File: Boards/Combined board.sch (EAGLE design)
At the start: 9 parts

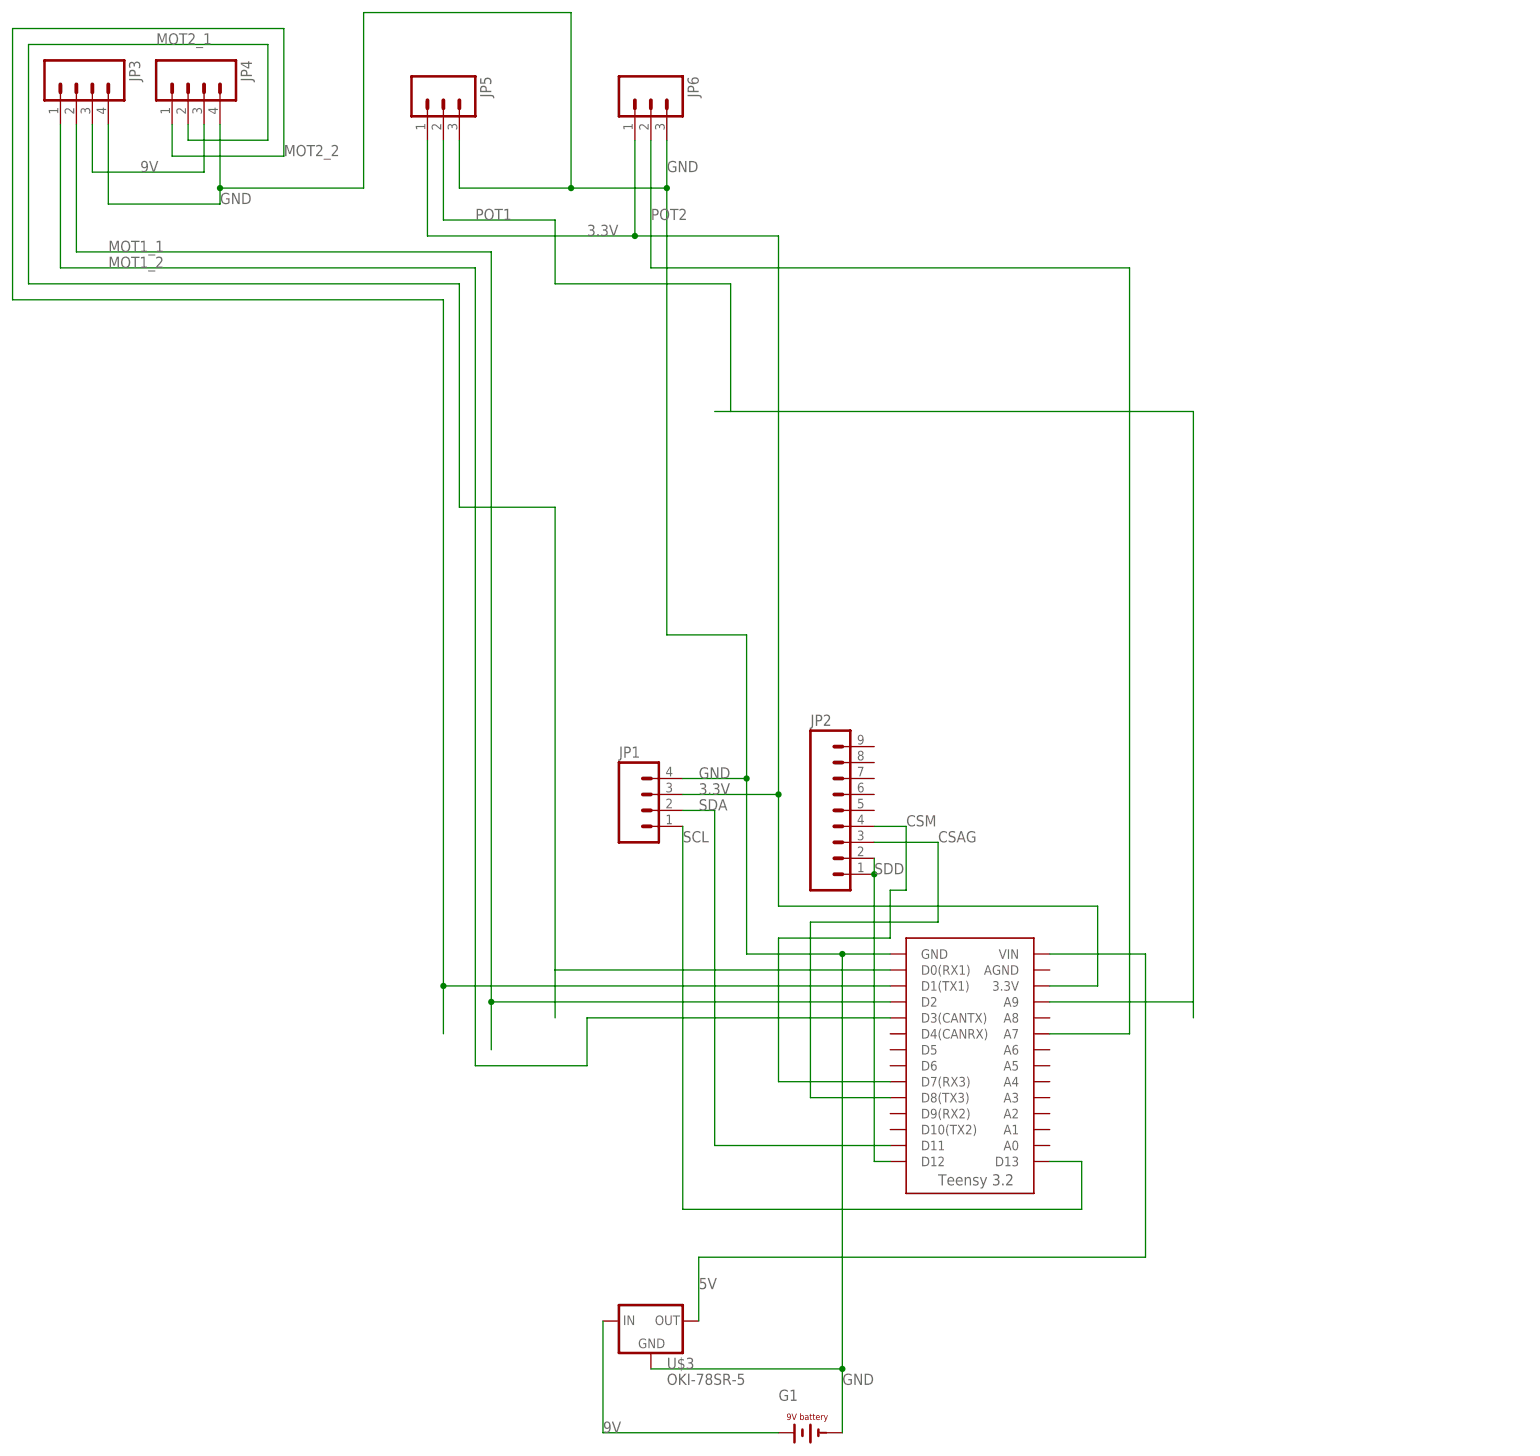
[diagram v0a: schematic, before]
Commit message: Final Push
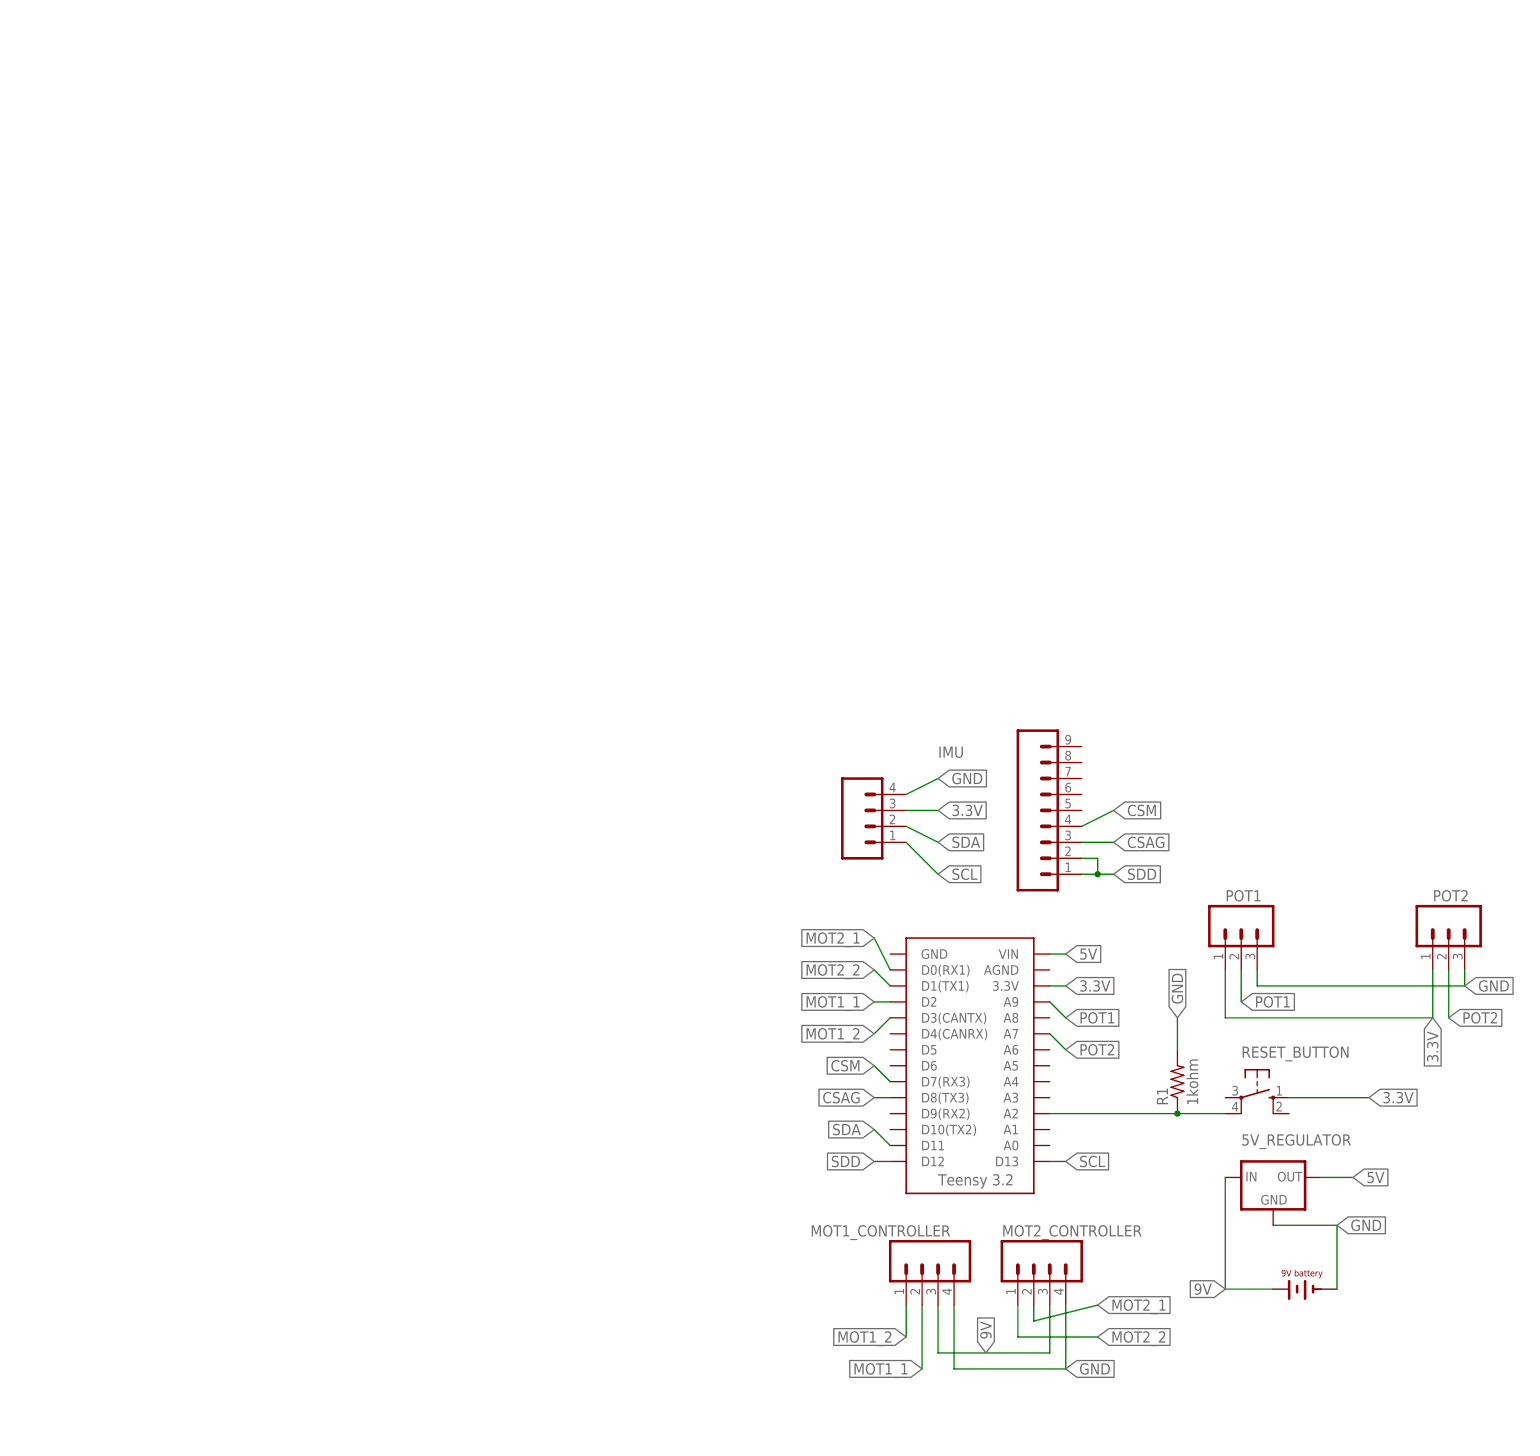
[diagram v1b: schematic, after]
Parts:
- removed JP2: (no value), HyTechDevices:M09
- removed JP3, JP4: (no value), HyTechDevices:M04
- removed JP5, JP6: (no value), HyTechDevices:M03
- removed U$3: OKI-78SR-5, HyTechDevices:OKI-78SR-5
- added 5V_REGULATOR: OKI-78SR-5, HyTechDevices:OKI-78SR-5
- added IMU: (no value), HyTechDevices:M09
- added MOT1_CONTROLLER, MOT2_CONTROLLER: (no value), HyTechDevices:M04
- added POT1, POT2: (no value), HyTechDevices:M03
- added R1: 1kohm, HyTechDevices:RESISTORAXIAL-0.3
- added RESET_BUTTON: (no value), HyTechDevices:BTN_10-XX
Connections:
- new net N$1: R1.1, RESET_BUTTON.P1, U$2.A2
- net 3.3V: now also POT1.1, POT2.1, RESET_BUTTON.S; no longer JP5.1, JP6.1
- net 5V: now also 5V_REGULATOR.OUT; no longer U$3.OUT
- net 9V: now also 5V_REGULATOR.IN, MOT1_CONTROLLER.3, MOT2_CONTROLLER.3; no longer JP3.3, JP4.3, U$3.IN
- net CSAG: now also IMU.3; no longer JP2.3
- net CSM: now also IMU.4; no longer JP2.4
- net GND: now also 5V_REGULATOR.GND, MOT1_CONTROLLER.4, MOT2_CONTROLLER.4, POT1.3, POT2.3, R1.2; no longer JP3.4, JP4.4, JP5.3, JP6.3, U$2.GND, U$3.GND
- net MOT1_1: now also MOT1_CONTROLLER.2; no longer JP3.2
- net MOT1_2: now also MOT1_CONTROLLER.1; no longer JP3.1
- net MOT2_1: now also MOT2_CONTROLLER.2; no longer JP4.2
- net MOT2_2: now also MOT2_CONTROLLER.1; no longer JP4.1
- net POT1: now also POT1.2; no longer JP5.2
- net POT2: now also POT2.2; no longer JP6.2
- net SDD: now also IMU.1, IMU.2; no longer JP2.1, JP2.2
